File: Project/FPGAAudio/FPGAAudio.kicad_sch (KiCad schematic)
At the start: 35 parts, among them J1 Conn_01x02_Pin, J2 Conn_01x08_Pin, SW1 SW_SPDT, SW2 SW_SPDT, U1 PAM8403D

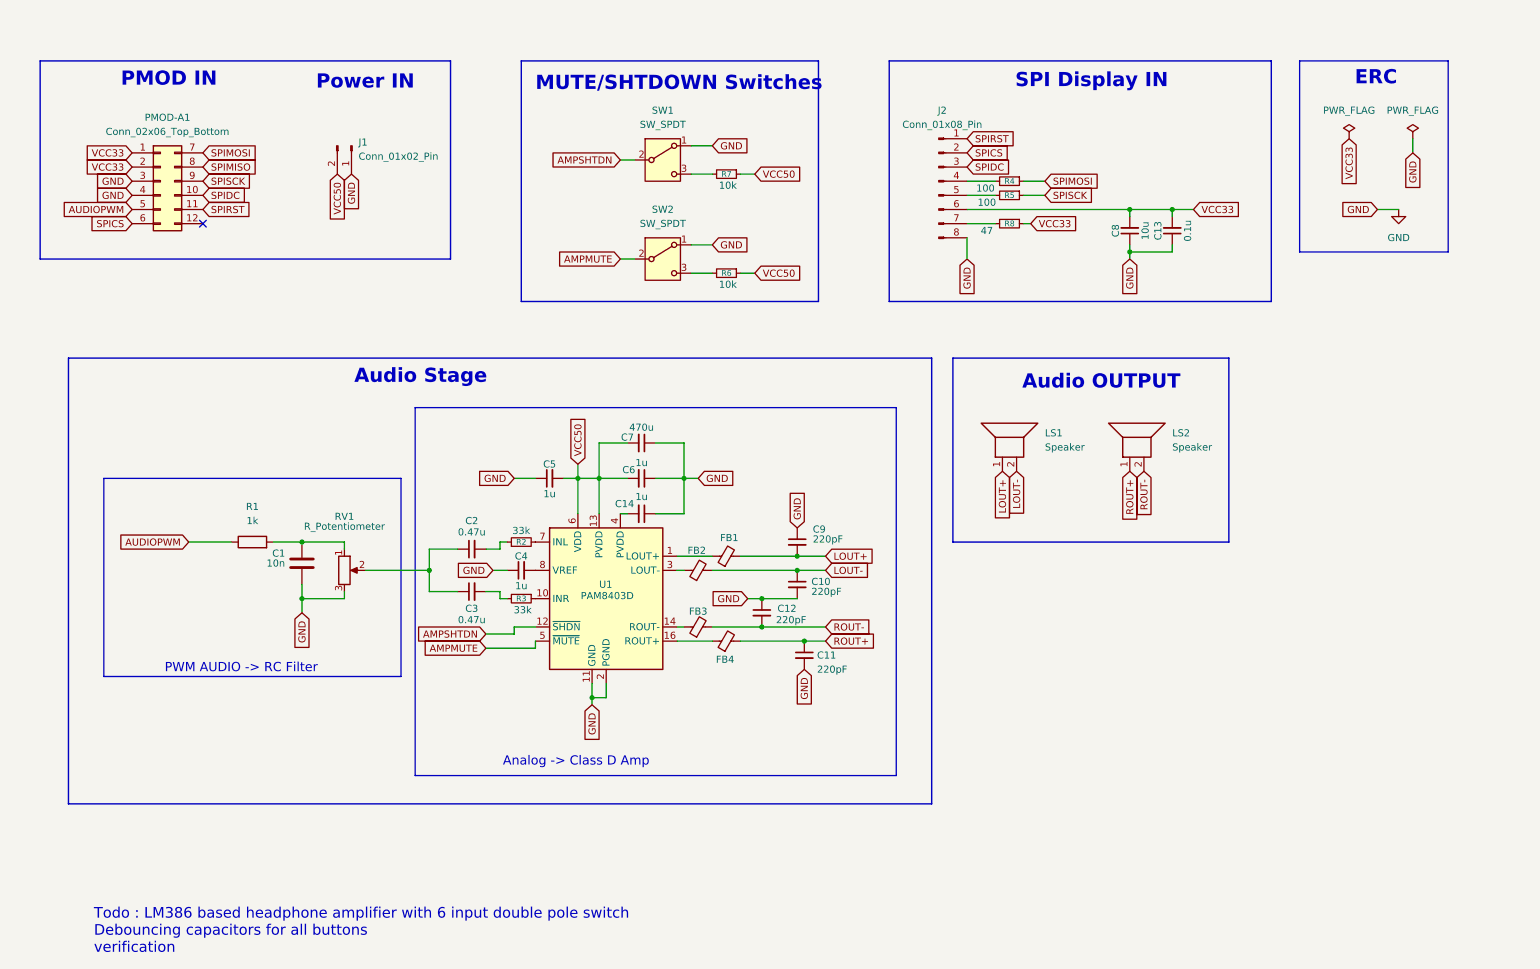
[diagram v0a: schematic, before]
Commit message: yeyeeye
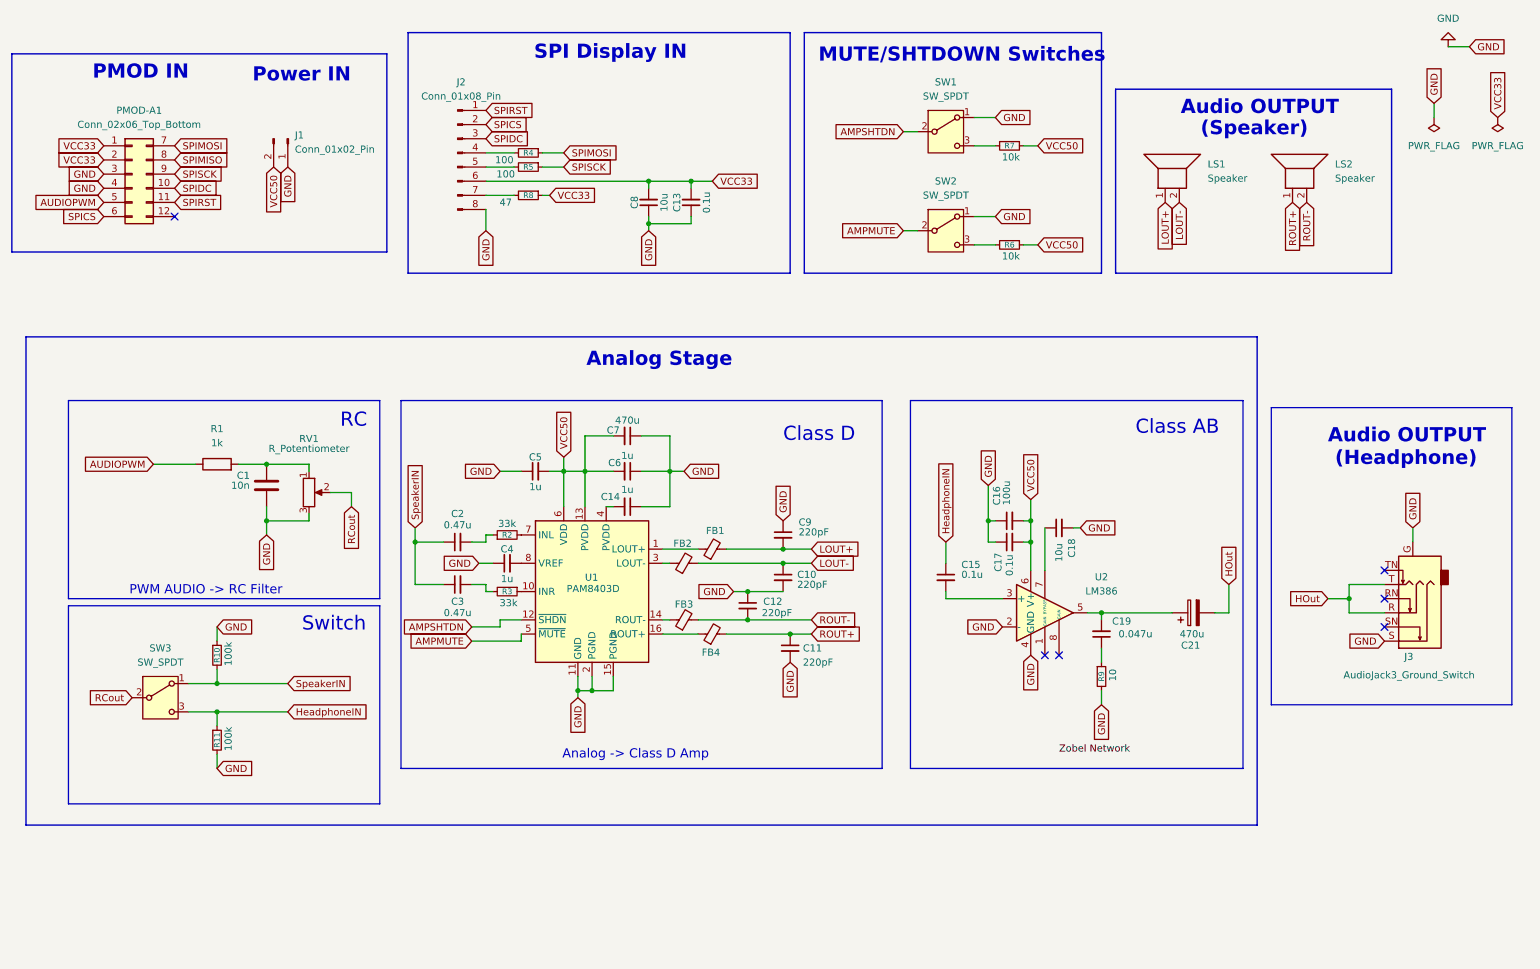
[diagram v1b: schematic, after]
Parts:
- added C15, C17: 0.1u, symbol Device:C_Small
- added C16: 100u, symbol Device:C_Small
- added C18: 10u, symbol Device:C_Small
- added C19: 0.047u, symbol Device:C_Small
- added C21: 470u, symbol Device:C_Polarized
- added J3: AudioJack3_Ground_Switch, symbol Connector_Audio:AudioJack3_Ground_Switch
- added R10, R11: 100k, symbol Device:R_Small
- added R9: 10, symbol Device:R_Small
- added SW3: SW_SPDT, symbol Switch:SW_SPDT
- added U2: LM386, symbol Amplifier_Audio:LM386
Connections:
- net GND: now also C16.1, C17.1, C18.2, J3.G, J3.S, R10.1, R11.2, R9.2, U2.2 (-), U2.4 (GND)
- net VCC50: now also C16.2, C17.2, U2.6 (V+)
- net SpeakerIN: now reaches C2.1, C3.1
- net SpeakerIN: now also R10.2, SW3.1 (A); no longer RV1.2
- new net: C15.2, U2.3 (+)
- new net: C19.2, C21.1, U2.5
- new net: C18.1, U2.7 (BYPASS)
- new net: C19.1, R9.1
- new net HOut: C21.2, J3.R, J3.T
- new net HeadphoneIN: C15.1, R11.1, SW3.3 (C)
- new net RCout: RV1.2, SW3.2 (B)
- no-connect marks 1 -> 6
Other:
- note added: "(Headphone)"
- note added: "(Speaker)"
- note added: "Analog Stage"
- note added: "Class AB"
- note added: "Class D"
- note added: "RC"
- note added: "Switch"
- note removed: "Audio Stage"
- note removed: "ERC"
- note removed: "Todo : LM386 based headphone amplifier with 6 input double pole switch Debouncing capacitors for all buttons verification"
- moved on the sheet: C1, C10, C11, C12, C13, C14, C2, C3, C4, C5, C6, C7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
